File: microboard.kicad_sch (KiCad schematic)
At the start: 92 parts, among them J10 Conn_01x01, J11 Conn_01x01, J12 Conn_01x10, J13 Conn_01x01, J14 Conn_01x12, J15 Conn_01x03, J17 Conn_01x01, J18 Conn_01x01, J2 Conn_01x10, J21 Conn_01x01_Socket, J22 Conn_01x01_Socket, J3 Conn_02x12, J39 Conn_01x10, J4 USB4085-GF-A_REVB, J40 Conn_01x10, J41 Conn_01x10, J43 Conn_01x05, J44 Conn_01x09, J45 Conn_01x08, J5 Conn_01x04, J6 Conn_01x04, J7 Conn_01x05, J8 Conn_01x10, J9 Conn_01x01, SW1 SW_Push, SW2 SW_Push, SW7 RotaryEncoder_Switch, U1 USBLC6-2SC6, U2 ATSAMD21G18A-AUT, U3 LF33_TO220, U7 LF50_TO220, Y1 32768Hz

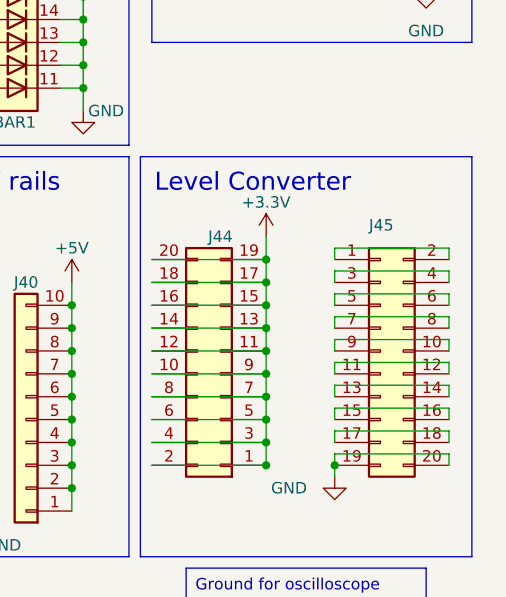
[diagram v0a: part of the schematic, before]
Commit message: final?
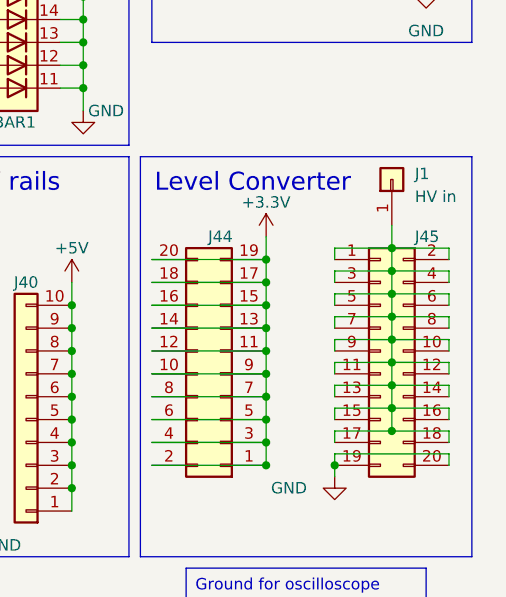
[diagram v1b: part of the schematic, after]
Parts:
- added J1: HV in, Connector_PinHeader_2.54mm:PinHeader_1x01_P2.54mm_Vertical, symbol Connector_Generic:Conn_01x01
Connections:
- net at J45.1 (Pin_1), J45.2 (Pin_2): now also J45.10 (Pin_10), J45.11 (Pin_11), J45.12 (Pin_12), J45.13 (Pin_13), J45.14 (Pin_14), J45.15 (Pin_15), J45.16 (Pin_16), J45.17 (Pin_17), J45.18 (Pin_18), J45.3 (Pin_3), J45.4 (Pin_4), J45.5 (Pin_5), J45.6 (Pin_6), J45.7 (Pin_7), J45.8 (Pin_8), J45.9 (Pin_9), J1.1 (Pin_1)
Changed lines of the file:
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@@
   (junction (at 241.3 40.64) (diameter 0) (color 0 0 0 0)
   )
+  (junction (at 275.59 68.58) (diameter 0) (color 0 0 0 0)
+  )
   (junction (at 144.78 154.94) (diameter 0) (color 0 0 0 0)
   )
   (junction (at 170.18 76.2) (diameter 0) (color 0 0 0 0)
   )
+  (junction (at 275.59 81.28) (diameter 0) (color 0 0 0 0)
+  )
   (junction (at 269.24 85.09) (diameter 0) (color 0 0 0 0)
   )
+  (junction (at 275.59 60.96) (diameter 0) (color 0 0 0 0)
+  )
   (junction (at 209.55 134.62) (diameter 0) (color 0 0 0 0)
   )
@@
   (junction (at 228.6 90.17) (diameter 0) (color 0 0 0 0)
   )
+  (junction (at 275.59 71.12) (diameter 0) (color 0 0 0 0)
+  )
   (junction (at 49.53 147.32) (diameter 0) (color 0 0 0 0)
   )
@@
   (junction (at 170.18 72.39) (diameter 0) (color 0 0 0 0)
   )
+  (junction (at 275.59 63.5) (diameter 0) (color 0 0 0 0)
+  )
   (junction (at 26.67 67.31) (diameter 0) (color 0 0 0 0)
   )
+  (junction (at 275.59 76.2) (diameter 0) (color 0 0 0 0)
+  )
   (junction (at 261.62 72.39) (diameter 0) (color 0 0 0 0)
   )
@@
   (junction (at 34.29 46.99) (diameter 0) (color 0 0 0 0)
   )
+  (junction (at 275.59 66.04) (diameter 0) (color 0 0 0 0)
+  )
   (junction (at 172.72 154.94) (diameter 0) (color 0 0 0 0)
   )
@@
   (junction (at 157.48 57.15) (diameter 0) (color 0 0 0 0)
   )
+  (junction (at 275.59 73.66) (diameter 0) (color 0 0 0 0)
+  )
   (junction (at 261.62 69.85) (diameter 0) (color 0 0 0 0)
   )
@@
   (junction (at 68.1593 177.4117) (diameter 0) (color 0 0 0 0)
   )
+  (junction (at 275.59 78.74) (diameter 0) (color 0 0 0 0)
+  )
   (junction (at 228.6 74.93) (diameter 0) (color 0 0 0 0)
   )
@@
     (stroke (width 0) (type default))
   )
+  (wire (pts (xy 275.59 60.96) (xy 275.59 63.5))
+    (stroke (width 0) (type default))
+  )
   (wire (pts (xy 147.32 123.19) (xy 157.48 123.19))
     (stroke (width 0) (type default))
   )
-  (wire (pts (xy 269.24 68.58) (xy 281.94 68.58))
+  (wire (pts (xy 275.59 66.04) (xy 275.59 68.58))
+    (stroke (width 0) (type default))
+  )
+  (wire (pts (xy 269.24 68.58) (xy 275.59 68.58))
     (stroke (width 0) (type default))
   )
@@
     (stroke (width 0) (type default))
   )
+  (wire (pts (xy 275.59 78.74) (xy 275.59 81.28))
+    (stroke (width 0) (type default))
+  )
+  (wire (pts (xy 275.59 73.66) (xy 275.59 76.2))
+    (stroke (width 0) (type default))
+  )
   (wire (pts (xy 48.26 96.52) (xy 48.26 95.25))
     (stroke (width 0) (type default))
@@
     (stroke (width 0) (type default))
   )
+  (wire (pts (xy 275.59 78.74) (xy 281.94 78.74))
+    (stroke (width 0) (type default))
+  )
   (wire (pts (xy 48.26 85.09) (xy 35.56 85.09))
     (stroke (width 0) (type default))
@@
     (stroke (width 0) (type default))
   )
-  (wire (pts (xy 281.94 76.2) (xy 269.24 76.2))
+  (wire (pts (xy 281.94 76.2) (xy 275.59 76.2))
     (stroke (width 0) (type default))
   )
@@
     (stroke (width 0) (type default))
   )
-  (wire (pts (xy 281.94 71.12) (xy 269.24 71.12))
+  (wire (pts (xy 281.94 71.12) (xy 275.59 71.12))
     (stroke (width 0) (type default))
   )
@@
     (stroke (width 0) (type default))
   )
-  (wire (pts (xy 269.24 73.66) (xy 281.94 73.66))
+  (wire (pts (xy 269.24 73.66) (xy 275.59 73.66))
     (stroke (width 0) (type default))
   )
@@
     (stroke (width 0) (type default))
   )
+  (wire (pts (xy 275.59 71.12) (xy 269.24 71.12))
+    (stroke (width 0) (type default))
+  )
   (wire (pts (xy 102.4493 172.3317) (xy 102.4493 174.8717))
     (stroke (width 0) (type default))
@@
     (stroke (width 0) (type default))
   )
+  (wire (pts (xy 275.59 60.96) (xy 269.24 60.96))
+    (stroke (width 0) (type default))
+  )
   (wire (pts (xy 165.1 139.7) (xy 165.1 135.89))
     (stroke (width 0) (type default))
@@
     (stroke (width 0) (type default))
   )
-  (wire (pts (xy 281.94 60.96) (xy 269.24 60.96))
+  (wire (pts (xy 281.94 60.96) (xy 275.59 60.96))
     (stroke (width 0) (type default))
   )
@@
     (stroke (width 0) (type default))
   )
-  (wire (pts (xy 281.94 66.04) (xy 269.24 66.04))
+  (wire (pts (xy 281.94 66.04) (xy 275.59 66.04))
     (stroke (width 0) (type default))
   )
@@
     (stroke (width 0) (type default))
   )
+  (wire (pts (xy 275.59 73.66) (xy 281.94 73.66))
+    (stroke (width 0) (type default))
+  )
   (wire (pts (xy 64.3493 144.3917) (xy 64.3493 169.7917))
     (stroke (width 0) (type default))
@@
     (stroke (width 0) (type default))
   )
+  (wire (pts (xy 275.59 71.12) (xy 275.59 73.66))
+    (stroke (width 0) (type default))
+  )
   (wire (pts (xy 153.67 100.33) (xy 153.67 110.49))
     (stroke (width 0) (type default))
@@
     (stroke (width 0) (type default))
   )
+  (wire (pts (xy 275.59 76.2) (xy 275.59 78.74))
+    (stroke (width 0) (type default))
+  )
   (wire (pts (xy 48.26 88.9) (xy 48.26 87.63))
     (stroke (width 0) (type default))
@@
     (stroke (width 0) (type default))
   )
+  (wire (pts (xy 275.59 76.2) (xy 269.24 76.2))
+    (stroke (width 0) (type default))
+  )
   (wire (pts (xy 252.73 127) (xy 261.62 127))
     (stroke (width 0) (type default))
@@
     (stroke (width 0) (type default))
   )
+  (wire (pts (xy 275.59 63.5) (xy 275.59 66.04))
+    (stroke (width 0) (type default))
+  )
   (wire (pts (xy 157.48 127) (xy 170.18 127))
     (stroke (width 0) (type default))
@@
     (stroke (width 0) (type default))
   )
-  (wire (pts (xy 281.94 81.28) (xy 269.24 81.28))
+  (wire (pts (xy 281.94 81.28) (xy 275.59 81.28))
     (stroke (width 0) (type default))
   )
@@
     (stroke (width 0) (type default))
   )
-  (wire (pts (xy 269.24 78.74) (xy 281.94 78.74))
+  (wire (pts (xy 269.24 78.74) (xy 275.59 78.74))
     (stroke (width 0) (type default))
   )
@@
     (stroke (width 0) (type default))
   )
-  (wire (pts (xy 269.24 63.5) (xy 281.94 63.5))
+  (wire (pts (xy 269.24 63.5) (xy 275.59 63.5))
     (stroke (width 0) (type default))
   )
@@
     (stroke (width 0) (type default))
   )
+  (wire (pts (xy 275.59 66.04) (xy 269.24 66.04))
+    (stroke (width 0) (type default))
+  )
   (wire (pts (xy 281.94 68.58) (xy 281.94 69.85))
     (stroke (width 0) (type default))
@@
     (stroke (width 0) (type default))
   )
+  (wire (pts (xy 275.59 68.58) (xy 275.59 71.12))
+    (stroke (width 0) (type default))
+  )
   (wire (pts (xy 217.17 85.09) (xy 217.17 87.63))
     (stroke (width 0) (type default))
@@
     (stroke (width 0) (type default))
   )
+  (wire (pts (xy 275.59 68.58) (xy 281.94 68.58))
+    (stroke (width 0) (type default))
+  )
   (wire (pts (xy 170.18 114.3) (xy 170.18 115.57))
     (stroke (width 0) (type default))
@@
     (stroke (width 0) (type default))
   )
+  (wire (pts (xy 275.59 63.5) (xy 281.94 63.5))
+    (stroke (width 0) (type default))
+  )
   (wire (pts (xy 228.6 67.31) (xy 228.6 69.85))
     (stroke (width 0) (type default))
@@
     (stroke (width 0) (type default))
   )
+  (wire (pts (xy 275.59 81.28) (xy 269.24 81.28))
+    (stroke (width 0) (type default))
+  )
   (wire (pts (xy 68.1593 177.4117) (xy 68.1593 181.7285))
     (stroke (width 0) (type default))
   )
+  (wire (pts (xy 275.59 58.42) (xy 275.59 60.96))
+    (stroke (width 0) (type default))
+  )
   (wire (pts (xy 146.05 87.63) (xy 146.05 95.25))
     (stroke (width 0) (type default))
@@
     )
   )
+  (symbol (lib_id "Connector_Generic:Conn_01x01") (at 275.59 53.34 90) (unit 1)
+    (in_bom yes) (on_board yes) (dnp no) (fields_autoplaced)
+    (property "Reference" "J1" (at 278.13 52.705 90)
+      (effects (font (size 1.27 1.27)) (justify right))
+    )
+    (property "Value" "HV in " (at 278.13 55.245 90)
+      (effects (font (size 1.27 1.27)) (justify right))
+    )
+    (property "Footprint" "Connector_PinHeader_2.54mm:PinHeader_1x01_P2.54mm_Vertical" (at 275.59 53.34 0)
+      (effects (font (size 1.27 1.27)) hide)
+    )
+    (property "Datasheet" "~" (at 275.59 53.34 0)
+      (effects (font (size 1.27 1.27)) hide)
+    )
+    (pin "1")
+    (instances
+      (project "microboard"
+        (path "/967dc07d-fccd-440b-a2b8-2bc1d125ec48"
+          (reference "J1") (unit 1)
+        )
+      )
+    )
+  )
   (symbol (lib_id "power:+3.3V") (at 15.24 55.88 0) (unit 1)
     (in_bom yes) (on_board yes) (dnp no) (fields_autoplaced)
@@
   (symbol (lib_id "Connector_Generic:Conn_02x10_Odd_Even") (at 274.32 72.39 0) (unit 1)
     (in_bom yes) (on_board yes) (dnp no)
-    (property "Reference" "J45" (at 273.05 58.42 0)
+    (property "Reference" "J45" (at 278.13 59.69 0)
       (effects (font (size 1.27 1.27)) (justify left))
     )
